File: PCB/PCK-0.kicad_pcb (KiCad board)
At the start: 4 copper layers, 166.7 x 78 mm, 86 parts, among them J1 USB_C_Receptacle_USB2.0_16P, SW1 EN, SW10 7,1, SW11 1,2, SW12 2,2, SW13 3,2, SW14 4,2, SW15 5,2, SW16 6,2, SW17 7,2, SW18 1,3, SW19 2,3, SW2 BOOT, SW20 3,3, SW21 4,3, SW22 5,3, SW23 6,3, SW24 7,3, SW25 1,4, SW26 2,4, SW27 3,4, SW28 4,4, SW29 5,4, SW3 RotaryEncoder_Switch_MP, SW30 6,4, SW31 7,4, SW4 1,1, SW5 2,1, SW6 3,1, SW7 4,1, SW8 5,1, SW9 6,1, U1 NCP1117-3.3_SOT223, U2 NCP1117-3.3_SOT223, U3 USBLC6-2SC6, U4 ESP32-C6-MINI-1, U5 TVS1400DRV

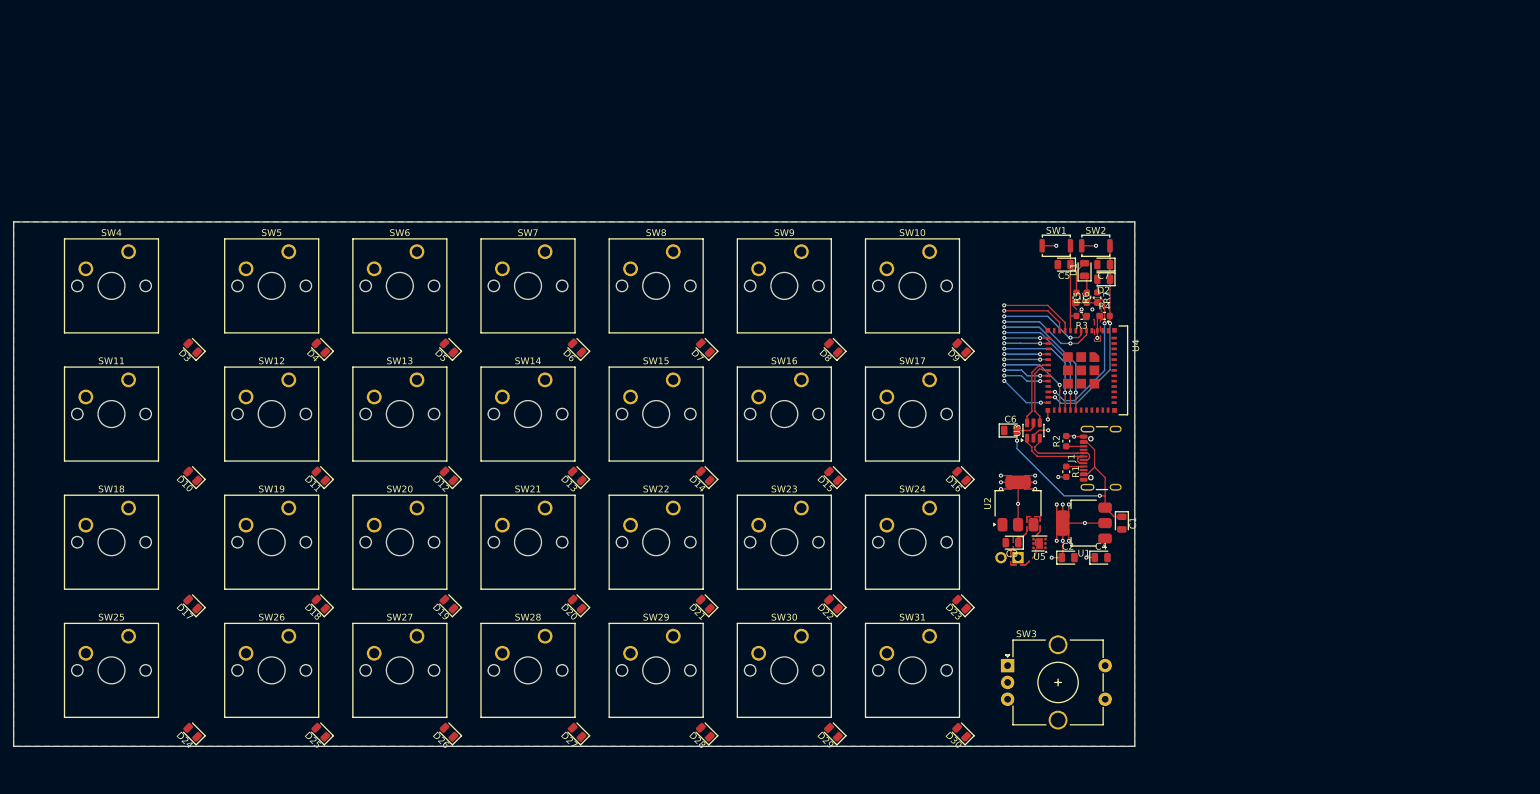
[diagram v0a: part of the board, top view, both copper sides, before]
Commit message: reformat + modular control scheme
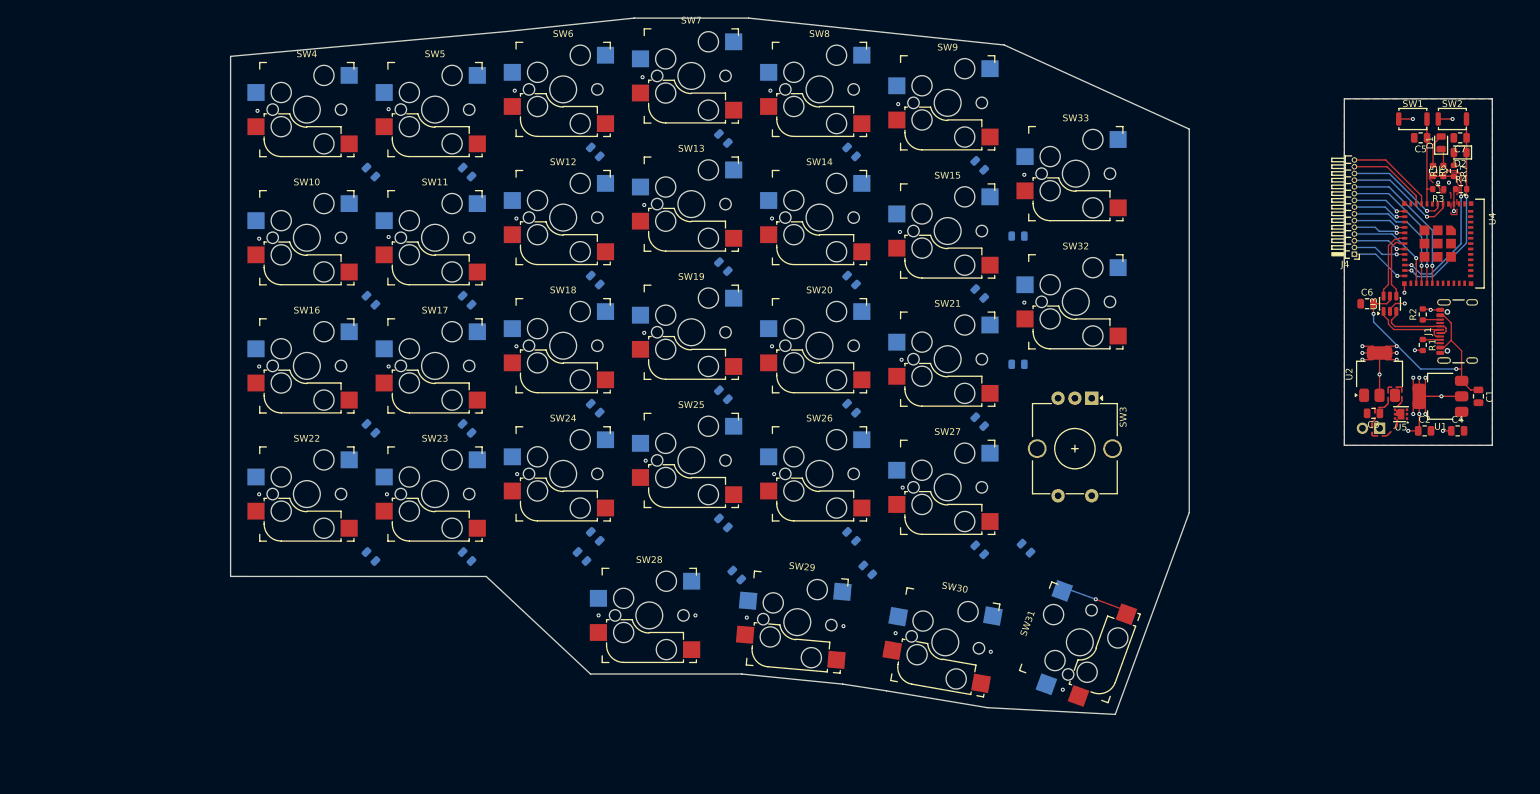
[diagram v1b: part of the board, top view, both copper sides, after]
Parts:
- removed the D16 at (130.7, 92.6)
- removed the D23 at (130.7, 111.6)
- removed the D9 at (130.7, 73.5)
- removed the SW10 at (125.9, 59.2)
- removed the SW17 at (125.9, 78.3)
- removed the SW24 at (125.9, 97.3)
- added D27: D, Diode_SMD:D_0805_2012Metric, B.Cu at (74.2, 104.5)
- added D28: D, Diode_SMD:D_0805_2012Metric, B.Cu at (97.2, 107.3)
- added D29: D, Diode_SMD:D_0805_2012Metric, B.Cu at (116.7, 106.5)
- added D31: D, Diode_SMD:D_0805_2012Metric, B.Cu at (139.1, 76.0)
- added D32: D, Diode_SMD:D_0805_2012Metric, B.Cu at (139.1, 56.9)
- added J4: Conn_01x15, Connector_PinHeader_1.00mm:PinHeader_1x15_P1.00mm_Horizontal, F.Cu at (189.1, 59.6)
- added SW28: 1,4, kb_switch:Kailh_socket_MX_reversible, F.Cu at (84.2, 113.3)
- added SW29: 2,4, kb_switch:Kailh_socket_MX_reversible, F.Cu at (106.2, 114.3)
- added SW30: 3,4, kb_switch:Kailh_socket_MX_reversible, F.Cu at (128.2, 117.3)
- added SW32: 5,4, kb_switch:Kailh_socket_MX_reversible, F.Cu at (147.6, 66.7)
- added SW33: 6,4, kb_switch:Kailh_socket_MX_reversible, F.Cu at (147.6, 47.6)
- C1, C2, C3, C4, C5, C6, C7: footprint Diode_SMD:D_0805_2012Metric -> Capacitor_SMD:C_0805_2012Metric
- D10: renamed from D11; moved to B.Cu
- D11: renamed from D12; moved to B.Cu
- D12: renamed from D13; moved to B.Cu
- D13: renamed from D14; moved to B.Cu
- D14: renamed from D15; moved to B.Cu
- D15: renamed from D17; moved to B.Cu
- D16: renamed from D18; moved to B.Cu
- D17: renamed from D19; moved to B.Cu
- D18: renamed from D20; moved to B.Cu
- D19: renamed from D21; moved to B.Cu
- D20: renamed from D22; moved to B.Cu
- D21: renamed from D24; moved to B.Cu
- D22: renamed from D25; moved to B.Cu
- D23: renamed from D26; moved to B.Cu
- D24: renamed from D27; moved to B.Cu
- D25: renamed from D28; moved to B.Cu
- D26: renamed from D29; moved to B.Cu
- D3, D30, D4, D5, D6, D7, D8: moved to B.Cu
- D9: renamed from D10; moved to B.Cu
- R1, R2, R3, R4, R5, R6, R7: footprint Capacitor_SMD:C_0603_1608Metric -> Resistor_SMD:R_0603_1608Metric
- SW10: renamed from SW11; footprint Button_Switch_Keyboard:SW_Cherry_MX_1.50u_PCB -> kb_switch:Kailh_socket_MX_reversible
- SW11: renamed from SW12; footprint Button_Switch_Keyboard:SW_Cherry_MX_1.00u_PCB -> kb_switch:Kailh_socket_MX_reversible
- SW12: renamed from SW13; footprint Button_Switch_Keyboard:SW_Cherry_MX_1.00u_PCB -> kb_switch:Kailh_socket_MX_reversible
- SW13: renamed from SW14; footprint Button_Switch_Keyboard:SW_Cherry_MX_1.00u_PCB -> kb_switch:Kailh_socket_MX_reversible
- SW14: renamed from SW15; footprint Button_Switch_Keyboard:SW_Cherry_MX_1.00u_PCB -> kb_switch:Kailh_socket_MX_reversible
- SW15: renamed from SW16; footprint Button_Switch_Keyboard:SW_Cherry_MX_1.00u_PCB -> kb_switch:Kailh_socket_MX_reversible
- SW16: renamed from SW18; footprint Button_Switch_Keyboard:SW_Cherry_MX_1.50u_PCB -> kb_switch:Kailh_socket_MX_reversible
- SW17: renamed from SW19; footprint Button_Switch_Keyboard:SW_Cherry_MX_1.00u_PCB -> kb_switch:Kailh_socket_MX_reversible
- SW18: renamed from SW20; footprint Button_Switch_Keyboard:SW_Cherry_MX_1.00u_PCB -> kb_switch:Kailh_socket_MX_reversible
- SW19: renamed from SW21; footprint Button_Switch_Keyboard:SW_Cherry_MX_1.00u_PCB -> kb_switch:Kailh_socket_MX_reversible
- SW20: renamed from SW22; footprint Button_Switch_Keyboard:SW_Cherry_MX_1.00u_PCB -> kb_switch:Kailh_socket_MX_reversible
- SW21: renamed from SW23; footprint Button_Switch_Keyboard:SW_Cherry_MX_1.00u_PCB -> kb_switch:Kailh_socket_MX_reversible
- SW22: renamed from SW25; footprint Button_Switch_Keyboard:SW_Cherry_MX_1.50u_PCB -> kb_switch:Kailh_socket_MX_reversible
- SW23: renamed from SW26; footprint Button_Switch_Keyboard:SW_Cherry_MX_1.00u_PCB -> kb_switch:Kailh_socket_MX_reversible
- SW24: renamed from SW27; footprint Button_Switch_Keyboard:SW_Cherry_MX_1.00u_PCB -> kb_switch:Kailh_socket_MX_reversible
- SW25: renamed from SW28; footprint Button_Switch_Keyboard:SW_Cherry_MX_1.00u_PCB -> kb_switch:Kailh_socket_MX_reversible
- SW26: renamed from SW29; footprint Button_Switch_Keyboard:SW_Cherry_MX_1.00u_PCB -> kb_switch:Kailh_socket_MX_reversible
- SW27: renamed from SW30; footprint Button_Switch_Keyboard:SW_Cherry_MX_1.00u_PCB -> kb_switch:Kailh_socket_MX_reversible
- SW31: value 7,4 -> 4,4; footprint Button_Switch_Keyboard:SW_Cherry_MX_1.00u_PCB -> kb_switch:Kailh_socket_MX_reversible
- SW4: footprint Button_Switch_Keyboard:SW_Cherry_MX_1.50u_PCB -> kb_switch:Kailh_socket_MX_reversible
- SW5, SW6, SW7, SW8, SW9: footprint Button_Switch_Keyboard:SW_Cherry_MX_1.00u_PCB -> kb_switch:Kailh_socket_MX_reversible
- moved BT1 57.1 mm to (192.8, 85.5)
- moved U2 57.1 mm to (192.8, 77.4)
- moved C3 57.1 mm to (191.9, 83.2)
- moved U5 57.1 mm to (196.0, 83.4)
- moved C1 56.2 mm to (207.5, 80.7)
- moved C2 56.2 mm to (199.5, 85.9)
- moved C4 56.2 mm to (204.4, 85.9)
- moved C5 56.2 mm to (198.9, 42.3)
- moved C6 56.2 mm to (190.9, 67.0)
- moved C7 56.2 mm to (204.8, 42.3)
- moved D1 56.2 mm to (201.9, 43.0)
- moved D2 56.2 mm to (204.8, 44.5)
- moved J1 56.2 mm to (205.5, 71.1)
- moved R1 56.2 mm to (199.2, 73.1)
- moved R2 56.2 mm to (199.2, 68.5)
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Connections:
- D10 pad 1: /IO21 -> /IO1
- D11 pad 1: /IO21 -> /IO1
- D12 pad 1: /IO21 -> /IO1
- D13 pad 1: /IO21 -> /IO1
- D14 pad 1: /IO21 -> /IO1
- D15 pad 1: /IO6 -> /IO21
- D16 pad 1: /IO6 -> /IO21
- D17 pad 1: /IO6 -> /IO21
- D18 pad 1: /IO6 -> /IO21
- D19 pad 1: /IO6 -> /IO21
- D20 pad 1: /IO6 -> /IO21
- D21 pad 1: /IO7 -> /IO6
- D22 pad 1: /IO7 -> /IO6
- D23 pad 1: /IO7 -> /IO6
- D24 pad 1: /IO7 -> /IO6
- D25 pad 1: /IO7 -> /IO6
- D26 pad 1: /IO7 -> /IO6
- D3 pad 1: /IO1 -> /IO0
- D4 pad 1: /IO1 -> /IO0
- D5 pad 1: /IO1 -> /IO0
- D6 pad 1: /IO1 -> /IO0
- D7 pad 1: /IO1 -> /IO0
- D8 pad 1: /IO1 -> /IO0
- D9 pad 1: /IO21 -> /IO1
- SW3 pad A: /IO12 -> /IO20
- SW3 pad B: /IO14 -> /IO15
- SW3 pad C: /IO13 -> /IO14
- SW3 pad S1: /IO15 -> /IO18
- SW31 pad 1: /IO0 -> /IO2
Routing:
- net /IO23: track 19.8 -> 22.1 mm, vias 2 -> 1
- net /IO3: track 13.5 -> 15.7 mm
- net /IO4: track 11.3 -> 13.4 mm
- net /IO22: track 18.7 -> 20.8 mm, vias 2 -> 1
- net /IO5: track 10.2 -> 12.2 mm
- net /IO2: track 14.7 -> 16.6 mm
- net /IO0: track 6.55 -> 8.16 mm, vias 2 -> 1
- net /IO1: track 6.55 -> 8.08 mm, vias 2 -> 1
- net /IO21: track 16.9 -> 18.3 mm, vias 2 -> 1
- net /IO6: track 6.55 -> 7.91 mm, vias 2 -> 1
- net /IO7: track 6.55 -> 7.83 mm, vias 2 -> 1
- net /IO20: track 13.2 -> 14.4 mm, vias 2 -> 1
- net /IO14: track 6.88 -> 7.99 mm, vias 2 -> 1
- net /IO15: track 6.88 -> 7.91 mm, vias 2 -> 1
- net /IO18: track 7.87 -> 8.82 mm, vias 2 -> 1
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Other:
- board size 166.7 x 78 mm -> 187.6 x 103.5 mm

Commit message: double sided probably works
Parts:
- D10, D11, D12, D13, D14, D15, D16, D17, D18, D19, D20, D21, D22, D23, D24, D25, D26, D27, D28, D29, D3, D30, D31, D32, D4, D5, D6, D7, D8, D9: footprint Diode_SMD:D_0805_2012Metric -> Diode_THT:D_A-405_P2.54mm_Vertical_AnodeUp
- SW10, SW11, SW12, SW13, SW14, SW15, SW16, SW17, SW18, SW19, SW20, SW21, SW22, SW23, SW24, SW25, SW26, SW27, SW28, SW29, SW30, SW31, SW32, SW33, SW4, SW5, SW6, SW7, SW8, SW9: footprint kb_switch:Kailh_socket_MX_reversible -> KB_SWITCH:SW_MX_reversible
- moved C6 138.9 mm to (325.8, 33.5)
- moved D1 138.9 mm to (336.8, 9.59)
- moved R3 138.9 mm to (336.4, 16.5)
- moved U4 138.9 mm to (336.3, 24.6)
- moved C3 138.9 mm to (326.7, 49.8)
- moved C4 138.9 mm to (339.2, 52.4)
- moved C5 138.9 mm to (333.7, 8.85)
- moved C7 138.9 mm to (339.6, 8.85)
- moved D2 138.9 mm to (339.6, 11.0)
- moved J1 138.9 mm to (340.3, 37.6)
- moved R1 138.9 mm to (334.1, 39.6)
- moved R2 138.9 mm to (334.1, 35.1)
- moved R4 138.9 mm to (339.8, 16.5)
- moved R5 138.9 mm to (337.1, 13.8)
- moved R7 138.9 mm to (338.7, 13.8)
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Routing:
- net /IO3: vias 2 -> 1
- net /IO4: vias 1 -> 0
- net /IO5: vias 1 -> 0
- net /IO2: vias 2 -> 1
- net Net-(D9-A): vias 1 -> 0
- net Net-(D8-A): vias 1 -> 0
- net Net-(D7-A): vias 1 -> 0
- net Net-(D6-A): vias 1 -> 0
- net Net-(D5-A): vias 1 -> 0
- net Net-(D4-A): vias 1 -> 0
- net Net-(D32-A): vias 1 -> 0
- net Net-(D31-A): vias 1 -> 0
- net Net-(D30-A): vias 1 -> 0
- net Net-(D3-A): vias 1 -> 0
- net Net-(D29-A): vias 1 -> 0
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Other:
- board size 187.6 x 103.5 mm -> 321.9 x 127 mm
